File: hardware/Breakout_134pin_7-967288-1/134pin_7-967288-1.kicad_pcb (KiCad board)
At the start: 2 copper layers, 1 part

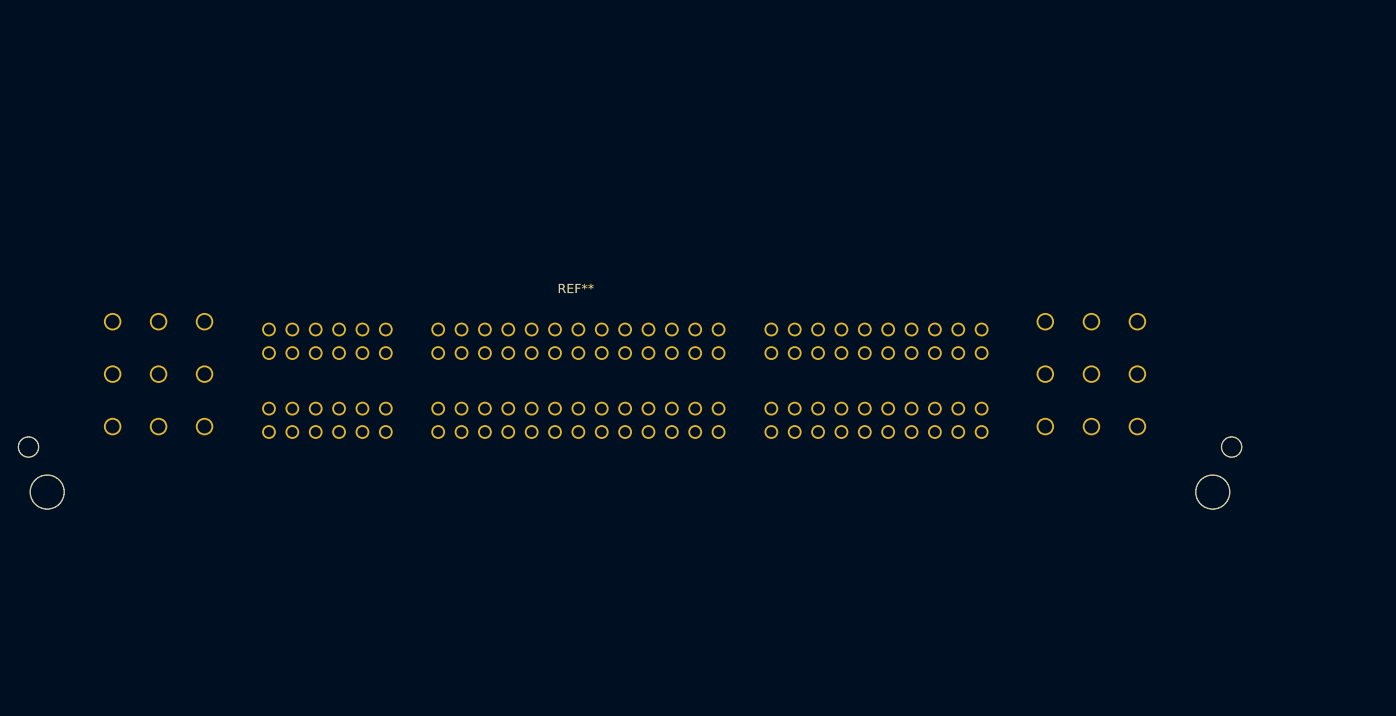
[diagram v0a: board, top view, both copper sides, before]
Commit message: 134 board
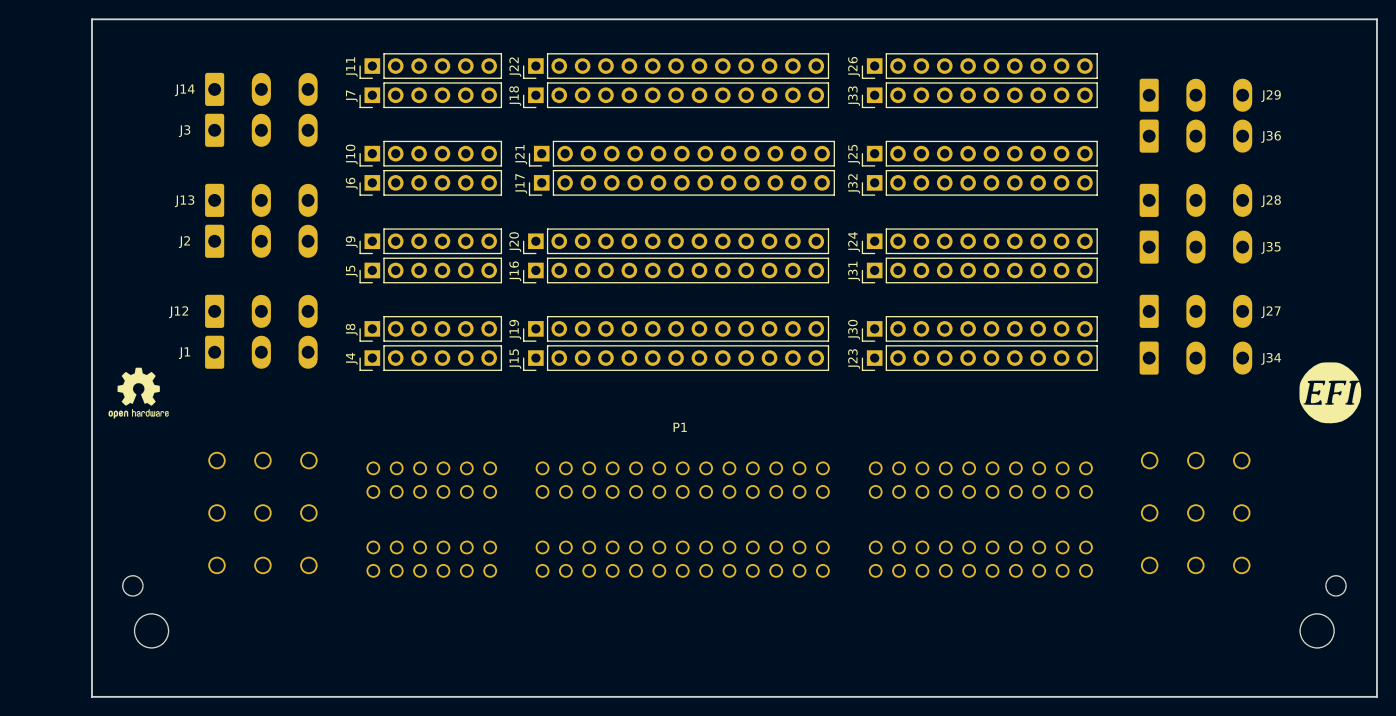
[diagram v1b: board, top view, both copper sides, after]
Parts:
- removed REF**: 7-967288-1_134-pin-connector, Breakout_134pin_7-967288-1_KC5:7-967288-1_134-pin-connector
- added J1: Conn_01x03, Connector_Phoenix_MSTB:PhoenixContact_MSTBA_2,5_3-G-5,08_1x03_P5.08mm_Horizontal, F.Cu at (89.5, 99.7)
- added J10: Conn_01x06, Connector_PinHeader_2.54mm:PinHeader_1x06_P2.54mm_Vertical, F.Cu at (106.7, 78.1)
- added J11: Conn_01x06, Connector_PinHeader_2.54mm:PinHeader_1x06_P2.54mm_Vertical, F.Cu at (106.7, 68.6)
- added J12: Conn_01x03, Connector_Phoenix_MSTB:PhoenixContact_MSTBA_2,5_3-G-5,08_1x03_P5.08mm_Horizontal, F.Cu at (89.5, 95.2)
- added J13: Conn_01x03, Connector_Phoenix_MSTB:PhoenixContact_MSTBA_2,5_3-G-5,08_1x03_P5.08mm_Horizontal, F.Cu at (89.5, 83.2)
- added J14: Conn_01x03, Connector_Phoenix_MSTB:PhoenixContact_MSTBA_2,5_3-G-5,08_1x03_P5.08mm_Horizontal, F.Cu at (89.5, 71.1)
- added J15: Conn_01x13, Connector_PinHeader_2.54mm:PinHeader_1x13_P2.54mm_Vertical, F.Cu at (124.5, 100.3)
- added J16: Conn_01x13, Connector_PinHeader_2.54mm:PinHeader_1x13_P2.54mm_Vertical, F.Cu at (124.5, 90.8)
- added J17: Conn_01x13, Connector_PinHeader_2.54mm:PinHeader_1x13_P2.54mm_Vertical, F.Cu at (125.1, 81.3)
- added J18: Conn_01x13, Connector_PinHeader_2.54mm:PinHeader_1x13_P2.54mm_Vertical, F.Cu at (124.5, 71.8)
- added J19: Conn_01x13, Connector_PinHeader_2.54mm:PinHeader_1x13_P2.54mm_Vertical, F.Cu at (124.5, 97.2)
- added J2: Conn_01x03, Connector_Phoenix_MSTB:PhoenixContact_MSTBA_2,5_3-G-5,08_1x03_P5.08mm_Horizontal, F.Cu at (89.5, 87.6)
- added J20: Conn_01x13, Connector_PinHeader_2.54mm:PinHeader_1x13_P2.54mm_Vertical, F.Cu at (124.5, 87.6)
- added J21: Conn_01x13, Connector_PinHeader_2.54mm:PinHeader_1x13_P2.54mm_Vertical, F.Cu at (125.1, 78.1)
- added J22: Conn_01x13, Connector_PinHeader_2.54mm:PinHeader_1x13_P2.54mm_Vertical, F.Cu at (124.5, 68.6)
- added J23: Conn_01x10, Connector_PinHeader_2.54mm:PinHeader_1x10_P2.54mm_Vertical, F.Cu at (161.3, 100.3)
- added J24: Conn_01x10, Connector_PinHeader_2.54mm:PinHeader_1x10_P2.54mm_Vertical, F.Cu at (161.3, 87.6)
- added J25: Conn_01x10, Connector_PinHeader_2.54mm:PinHeader_1x10_P2.54mm_Vertical, F.Cu at (161.3, 78.1)
- added J26: Conn_01x10, Connector_PinHeader_2.54mm:PinHeader_1x10_P2.54mm_Vertical, F.Cu at (161.3, 68.6)
- added J27: Conn_01x03, Connector_Phoenix_MSTB:PhoenixContact_MSTBA_2,5_3-G-5,08_1x03_P5.08mm_Horizontal, F.Cu at (191.1, 95.2)
- added J28: Conn_01x03, Connector_Phoenix_MSTB:PhoenixContact_MSTBA_2,5_3-G-5,08_1x03_P5.08mm_Horizontal, F.Cu at (191.1, 83.2)
- added J29: Conn_01x03, Connector_Phoenix_MSTB:PhoenixContact_MSTBA_2,5_3-G-5,08_1x03_P5.08mm_Horizontal, F.Cu at (191.1, 71.8)
- added J3: Conn_01x03, Connector_Phoenix_MSTB:PhoenixContact_MSTBA_2,5_3-G-5,08_1x03_P5.08mm_Horizontal, F.Cu at (89.5, 75.6)
- added J30: Conn_01x10, Connector_PinHeader_2.54mm:PinHeader_1x10_P2.54mm_Vertical, F.Cu at (161.3, 97.2)
- added J31: Conn_01x10, Connector_PinHeader_2.54mm:PinHeader_1x10_P2.54mm_Vertical, F.Cu at (161.3, 90.8)
- added J32: Conn_01x10, Connector_PinHeader_2.54mm:PinHeader_1x10_P2.54mm_Vertical, F.Cu at (161.3, 81.3)
- added J33: Conn_01x10, Connector_PinHeader_2.54mm:PinHeader_1x10_P2.54mm_Vertical, F.Cu at (161.3, 71.8)
- added J34: Conn_01x03, Connector_Phoenix_MSTB:PhoenixContact_MSTBA_2,5_3-G-5,08_1x03_P5.08mm_Horizontal, F.Cu at (191.1, 100.3)
- added J35: Conn_01x03, Connector_Phoenix_MSTB:PhoenixContact_MSTBA_2,5_3-G-5,08_1x03_P5.08mm_Horizontal, F.Cu at (191.1, 88.3)
- added J36: Conn_01x03, Connector_Phoenix_MSTB:PhoenixContact_MSTBA_2,5_3-G-5,08_1x03_P5.08mm_Horizontal, F.Cu at (191.1, 76.2)
- added J4: Conn_01x06, Connector_PinHeader_2.54mm:PinHeader_1x06_P2.54mm_Vertical, F.Cu at (106.7, 100.3)
- added J5: Conn_01x06, Connector_PinHeader_2.54mm:PinHeader_1x06_P2.54mm_Vertical, F.Cu at (106.7, 90.8)
- added J6: Conn_01x06, Connector_PinHeader_2.54mm:PinHeader_1x06_P2.54mm_Vertical, F.Cu at (106.7, 81.3)
- added J7: Conn_01x06, Connector_PinHeader_2.54mm:PinHeader_1x06_P2.54mm_Vertical, F.Cu at (106.7, 71.8)
- added J8: Conn_01x06, Connector_PinHeader_2.54mm:PinHeader_1x06_P2.54mm_Vertical, F.Cu at (106.7, 97.2)
- added J9: Conn_01x06, Connector_PinHeader_2.54mm:PinHeader_1x06_P2.54mm_Vertical, F.Cu at (106.7, 87.6)
- added LOGO1: DNP, rusEFI:LOGO, F.Cu at (210.8, 104.1)
- added LOGO2: DNP, Symbol:OSHW-Logo2_7.3x6mm_SilkScreen, F.Cu at (81.3, 104.1)
- added P1: 134pin_7-967288-1_KC5, 134pin_7-967288-1_KC5_FOOTPRINT:7-967288-1_134-pin-connector, F.Cu at (80.6, 125.1)
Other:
- board outline added: 139.7 x 73.7 mm
